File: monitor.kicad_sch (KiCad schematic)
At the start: 51 parts, among them J1 USB_C_Plug, J2 USB_C_Receptacle_USB2.0_14P, J3 Display, J4 Program, J5 Boot, U1 STM32U031K8Ux, U2 TPSM365R6V3RDNR, U3 TMP117xxDRV, U4 REF5025ADGK, U5 CC6903, Y1 32768Hz

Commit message: Manufacturing updates
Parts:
- J1, J2: now left out of the parts list
- R1: now in the parts list
- U4: JLCPCB C75881 -> C75881
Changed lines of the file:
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@@
 		(unit 1)
 		(exclude_from_sim no)
-		(in_bom yes)
+		(in_bom no)
 		(on_board yes)
 		(dnp no)
@@
 			)
 		)
-		(property "JLCPCB" " C75881"
+		(property "JLCPCB" "C75881"
 			(at 201.93 102.87 0)
 			(effects
@@
 		(unit 1)
 		(exclude_from_sim no)
-		(in_bom no)
+		(in_bom yes)
 		(on_board yes)
 		(dnp no)
@@
 		(unit 1)
 		(exclude_from_sim no)
-		(in_bom yes)
+		(in_bom no)
 		(on_board yes)
 		(dnp no)

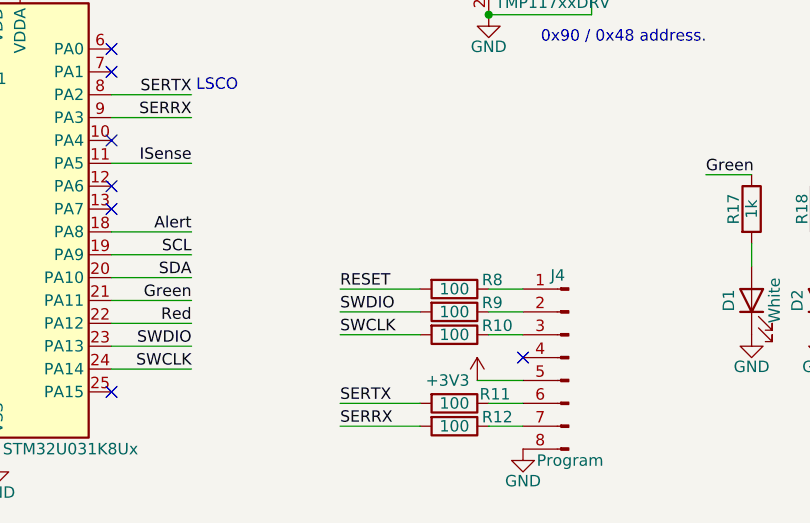
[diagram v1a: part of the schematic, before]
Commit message: Robustify reset
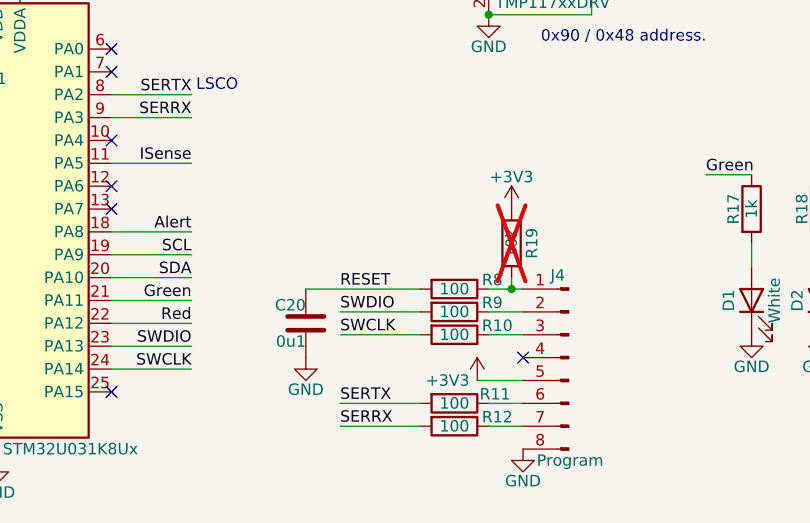
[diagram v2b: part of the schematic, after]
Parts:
- added C20: 0u1, Capacitor_SMD:C_0402_1005Metric, symbol Device:C
- added R19: 10k, Resistor_SMD:R_0603_1608Metric, symbol Device:R
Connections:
- net +3V3: now also R19.2
- net GND: now also C20.2
- net RESET: now also C20.1
- net at J4.1 (Pin_1), R8.1: now also R19.1
